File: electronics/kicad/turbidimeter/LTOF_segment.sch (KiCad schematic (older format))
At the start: 3 parts, among them U2 TSL2571FN

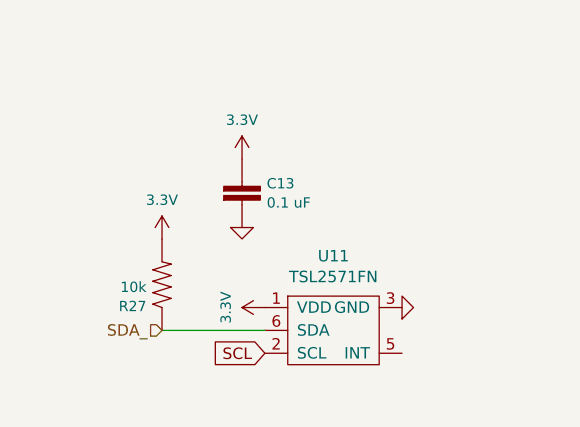
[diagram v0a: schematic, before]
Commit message: turbidimeter
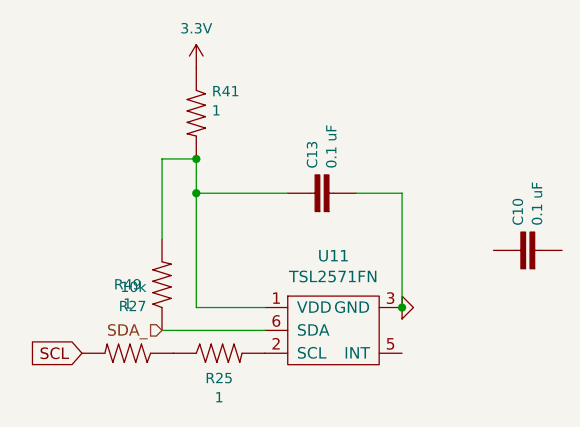
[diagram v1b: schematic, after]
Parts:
- added C3: 0.1 uF, Capacitor_SMD:C_0603_1608Metric, symbol SparkFun-Capacitors:0.1UF-0603-25V-5%
- added R23, R40, R48: 1, 0805, symbol SparkFun-Resistors:RESISTOR0805
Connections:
- net 3.3V: now also R40.1; no longer C4.1, R18.2, U2.1 (VDD)
- net SCL: now also R48.2; no longer U2.2 (SCL)
- new net: C4.1, R18.2, R40.2, U2.1 (VDD)
- new net: R23.2, U2.2 (SCL)
- new net: R23.1, R48.1
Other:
- moved on the sheet: C13
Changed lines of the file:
@@
 $Descr A4 11693 8268
 encoding utf-8
-Sheet 18 33
+Sheet 17 17
 Title ""
 Date ""
@@
 	1    0    0    -1
 $EndComp
-$Comp
-L SparkFun-PowerSymbols:3.3V #SUPPLY?
-U 1 1 5FC4995B
-P 3900 3850
-AR Path="/5FC4995B" Ref="#SUPPLY?"  Part="1"
-AR Path="/5FC47654/5FC4995B" Ref="#SUPPLY0107"  Part="1"
-AR Path="/5FC5771C/5FC4995B" Ref="#SUPPLY0108"  Part="1"
-AR Path="/5FC58972/5FC4995B" Ref="#SUPPLY0109"  Part="1"
-AR Path="/5FC5929A/5FC4995B" Ref="#SUPPLY0110"  Part="1"
-AR Path="/5FC59BFE/5FC4995B" Ref="#SUPPLY?"  Part="1"
-AR Path="/5FC5B14C/5FC4995B" Ref="#SUPPLY0111"  Part="1"
-AR Path="/5FC5B14F/5FC4995B" Ref="#SUPPLY0112"  Part="1"
-AR Path="/5FC5B152/5FC4995B" Ref="#SUPPLY0113"  Part="1"
-AR Path="/5FC5B155/5FC4995B" Ref="#SUPPLY0114"  Part="1"
-AR Path="/5FC5BFFA/5FC4995B" Ref="#SUPPLY0115"  Part="1"
-AR Path="/5FC5BFFD/5FC4995B" Ref="#SUPPLY0116"  Part="1"
-AR Path="/5FC5C000/5FC4995B" Ref="#SUPPLY0117"  Part="1"
-AR Path="/5FC5C003/5FC4995B" Ref="#SUPPLY0118"  Part="1"
-AR Path="/5FC5C006/5FC4995B" Ref="#SUPPLY0119"  Part="1"
-AR Path="/5FC5C009/5FC4995B" Ref="#SUPPLY0120"  Part="1"
-AR Path="/5FC5C00C/5FC4995B" Ref="#SUPPLY0121"  Part="1"
-AR Path="/5FC5C00F/5FC4995B" Ref="#SUPPLY0122"  Part="1"
-F 0 "#SUPPLY0116" H 3950 3850 45  0001 L BNN
-F 1 "3.3V" H 3900 4020 45  0000 C CNN
-F 2 "" V 3858 3977 60  0000 L CNN
-F 3 "" H 3900 3850 60  0001 C CNN
-	1    3900 3850
-	0    -1   -1   0
-$EndComp
-Text GLabel 3900 4050 0    50   Input ~ 0
+Text GLabel 3100 4050 0    50   Input ~ 0
 SCL
 $Comp
@@
 L SparkFun-PowerSymbols:3.3V #SUPPLY?
 U 1 1 5FCB8149
-P 3450 3550
+P 3600 2800
 AR Path="/5FCB8149" Ref="#SUPPLY?"  Part="1"
 AR Path="/5FC47654/5FCB8149" Ref="#SUPPLY0123"  Part="1"
@@
 AR Path="/5FC5C00C/5FCB8149" Ref="#SUPPLY0137"  Part="1"
 AR Path="/5FC5C00F/5FCB8149" Ref="#SUPPLY0138"  Part="1"
-F 0 "#SUPPLY0132" H 3500 3550 45  0001 L BNN
-F 1 "3.3V" H 3450 3720 45  0000 C CNN
-F 2 "" V 3408 3677 60  0000 L CNN
-F 3 "" H 3450 3550 60  0001 C CNN
-	1    3450 3550
+F 0 "#SUPPLY0132" H 3650 2800 45  0001 L BNN
+F 1 "3.3V" H 3600 2970 45  0000 C CNN
+F 2 "" V 3558 2927 60  0000 L CNN
+F 3 "" H 3600 2800 60  0001 C CNN
+	1    3600 2800
 	1    0    0    -1
 $EndComp
 Wire Wire Line
 	3900 3950 3450 3950
-$Comp
-L power:GND #PWR?
-U 1 1 5FCB9EE0
-P 3800 3500
-AR Path="/5FCB9EE0" Ref="#PWR?"  Part="1"
-AR Path="/5FC47654/5FCB9EE0" Ref="#PWR0141"  Part="1"
-AR Path="/5FC5771C/5FCB9EE0" Ref="#PWR0142"  Part="1"
-AR Path="/5FC58972/5FCB9EE0" Ref="#PWR0143"  Part="1"
-AR Path="/5FC5929A/5FCB9EE0" Ref="#PWR0144"  Part="1"
-AR Path="/5FC5B14C/5FCB9EE0" Ref="#PWR0145"  Part="1"
-AR Path="/5FC5B14F/5FCB9EE0" Ref="#PWR0146"  Part="1"
-AR Path="/5FC5B152/5FCB9EE0" Ref="#PWR0147"  Part="1"
-AR Path="/5FC5B155/5FCB9EE0" Ref="#PWR0148"  Part="1"
-AR Path="/5FC5BFFA/5FCB9EE0" Ref="#PWR0149"  Part="1"
-AR Path="/5FC5BFFD/5FCB9EE0" Ref="#PWR0150"  Part="1"
-AR Path="/5FC5C000/5FCB9EE0" Ref="#PWR0151"  Part="1"
-AR Path="/5FC5C003/5FCB9EE0" Ref="#PWR0152"  Part="1"
-AR Path="/5FC5C006/5FCB9EE0" Ref="#PWR0153"  Part="1"
-AR Path="/5FC5C009/5FCB9EE0" Ref="#PWR0154"  Part="1"
-AR Path="/5FC5C00C/5FCB9EE0" Ref="#PWR0155"  Part="1"
-AR Path="/5FC5C00F/5FCB9EE0" Ref="#PWR0156"  Part="1"
-F 0 "#PWR0150" H 3800 3500 30  0001 C CNN
-F 1 "GND" H 3800 3430 30  0001 C CNN
-F 2 "" H 3800 3500 50  0001 C CNN
-F 3 "" H 3800 3500 50  0001 C CNN
-	1    3800 3500
-	1    0    0    -1
-$EndComp
 $Comp
 L SparkFun-Capacitors:0.1UF-0603-25V-5% C?
 U 1 1 5FCB9EE7
-P 3800 3400
+P 4200 3350
 AR Path="/5FCB9EE7" Ref="C?"  Part="1"
 AR Path="/5FC47654/5FCB9EE7" Ref="C4"  Part="1"
@@
 AR Path="/5FC5C00C/5FCB9EE7" Ref="C18"  Part="1"
 AR Path="/5FC5C00F/5FCB9EE7" Ref="C19"  Part="1"
-F 0 "C13" H 3908 3492 45  0000 L CNN
-F 1 "0.1 uF" H 3908 3408 45  0000 L CNN
-F 2 "Capacitor_SMD:C_0603_1608Metric" H 3800 3650 20  0001 C CNN
-F 3 "" H 3800 3400 50  0001 C CNN
-F 4 "" H 3908 3366 60  0000 L CNN "Field4"
-	1    3800 3400
+F 0 "C13" H 4308 3442 45  0000 L CNN
+F 1 "0.1 uF" H 4308 3358 45  0000 L CNN
+F 2 "Capacitor_SMD:C_0603_1608Metric" H 4200 3600 20  0001 C CNN
+F 3 "" H 4200 3350 50  0001 C CNN
+F 4 "" H 4308 3316 60  0000 L CNN "Field4"
+	1    4200 3350
+	0    -1   -1   0
+$EndComp
+Wire Wire Line
+	3450 3550 3450 3200
+$Comp
+L SparkFun-Resistors:RESISTOR0805 R23
+U 1 1 60C85497
+P 3700 4050
+AR Path="/5FC5C00F/60C85497" Ref="R23"  Part="1"
+AR Path="/5FC5BFFA/60C85497" Ref="R10"  Part="1"
+AR Path="/5FC5C000/60C85497" Ref="R12"  Part="1"
+AR Path="/5FC5C003/60C85497" Ref="R14"  Part="1"
+AR Path="/5FC5C006/60C85497" Ref="R16"  Part="1"
+AR Path="/5FC5C009/60C85497" Ref="R19"  Part="1"
+AR Path="/5FC5C00C/60C85497" Ref="R21"  Part="1"
+AR Path="/5FC5BFFD/60C85497" Ref="R25"  Part="1"
+F 0 "R25" H 3700 3940 45  0000 C CNN
+F 1 "1" H 3700 3856 45  0000 C CNN
+F 2 "0805" H 3700 4200 20  0001 C CNN
+F 3 "" H 3700 4050 60  0001 C CNN
+F 4 " " H 3700 3761 60  0000 C CNN "Field4"
+	1    3700 4050
 	1    0    0    -1
 $EndComp
-$Comp
-L SparkFun-PowerSymbols:3.3V #SUPPLY?
-U 1 1 5FCB9F0F
-P 3800 3200
-AR Path="/5FCB9F0F" Ref="#SUPPLY?"  Part="1"
-AR Path="/5FC47654/5FCB9F0F" Ref="#SUPPLY0139"  Part="1"
-AR Path="/5FC5771C/5FCB9F0F" Ref="#SUPPLY0140"  Part="1"
-AR Path="/5FC58972/5FCB9F0F" Ref="#SUPPLY0141"  Part="1"
-AR Path="/5FC5929A/5FCB9F0F" Ref="#SUPPLY0142"  Part="1"
-AR Path="/5FC59BFE/5FCB9F0F" Ref="#SUPPLY?"  Part="1"
-AR Path="/5FC5B14C/5FCB9F0F" Ref="#SUPPLY0143"  Part="1"
-AR Path="/5FC5B14F/5FCB9F0F" Ref="#SUPPLY0144"  Part="1"
-AR Path="/5FC5B152/5FCB9F0F" Ref="#SUPPLY0145"  Part="1"
-AR Path="/5FC5B155/5FCB9F0F" Ref="#SUPPLY0146"  Part="1"
-AR Path="/5FC5BFFA/5FCB9F0F" Ref="#SUPPLY0147"  Part="1"
-AR Path="/5FC5BFFD/5FCB9F0F" Ref="#SUPPLY0148"  Part="1"
-AR Path="/5FC5C000/5FCB9F0F" Ref="#SUPPLY0149"  Part="1"
-AR Path="/5FC5C003/5FCB9F0F" Ref="#SUPPLY0150"  Part="1"
-AR Path="/5FC5C006/5FCB9F0F" Ref="#SUPPLY0151"  Part="1"
-AR Path="/5FC5C009/5FCB9F0F" Ref="#SUPPLY0152"  Part="1"
-AR Path="/5FC5C00C/5FCB9F0F" Ref="#SUPPLY0153"  Part="1"
-AR Path="/5FC5C00F/5FCB9F0F" Ref="#SUPPLY0154"  Part="1"
-F 0 "#SUPPLY0148" H 3850 3200 45  0001 L BNN
-F 1 "3.3V" H 3800 3370 45  0000 C CNN
-F 2 "" V 3758 3327 60  0000 L CNN
-F 3 "" H 3800 3200 60  0001 C CNN
-	1    3800 3200
-	1    0    0    -1
-$EndComp
+Wire Wire Line
+	3600 3850 3900 3850
+Wire Wire Line
+	4500 3850 4500 3350
+Wire Wire Line
+	4500 3350 4300 3350
+Wire Wire Line
+	3600 3350 3600 3850
+Connection ~ 3600 3350
+Wire Wire Line
+	4000 3350 3600 3350
+Wire Wire Line
+	3600 3200 3600 3350
+$Comp
+L SparkFun-Resistors:RESISTOR0805 R48
+U 1 1 60C907D0
+P 3300 4050
+AR Path="/5FC5C00F/60C907D0" Ref="R48"  Part="1"
+AR Path="/5FC5BFFA/60C907D0" Ref="R42"  Part="1"
+AR Path="/5FC5C000/60C907D0" Ref="R43"  Part="1"
+AR Path="/5FC5C003/60C907D0" Ref="R44"  Part="1"
+AR Path="/5FC5C006/60C907D0" Ref="R45"  Part="1"
+AR Path="/5FC5C009/60C907D0" Ref="R46"  Part="1"
+AR Path="/5FC5C00C/60C907D0" Ref="R47"  Part="1"
+AR Path="/5FC5BFFD/60C907D0" Ref="R49"  Part="1"
+F 0 "R49" H 3300 3750 45  0000 C CNN
+F 1 "1" H 3300 3834 45  0000 C CNN
+F 2 "0805" H 3300 4200 20  0001 C CNN
+F 3 "" H 3300 4050 60  0001 C CNN
+F 4 " " H 3300 3929 60  0000 C CNN "Field4"
+	1    3300 4050
+	-1   0    0    1
+$EndComp
+Wire Wire Line
+	3450 3200 3600 3200
+Connection ~ 4500 3850
+$Comp
+L SparkFun-Capacitors:0.1UF-0603-25V-5% C?
+U 1 1 60C96374
+P 5100 3600
+AR Path="/60C96374" Ref="C?"  Part="1"
+AR Path="/5FC47654/60C96374" Ref="C?"  Part="1"
+AR Path="/5FC5771C/60C96374" Ref="C?"  Part="1"
+AR Path="/5FC58972/60C96374" Ref="C?"  Part="1"
+AR Path="/5FC5929A/60C96374" Ref="C?"  Part="1"
+AR Path="/5FC5B14C/60C96374" Ref="C?"  Part="1"
+AR Path="/5FC5B14F/60C96374" Ref="C?"  Part="1"
+AR Path="/5FC5B152/60C96374" Ref="C?"  Part="1"
+AR Path="/5FC5B155/60C96374" Ref="C?"  Part="1"
+AR Path="/5FC5BFFA/60C96374" Ref="C3"  Part="1"
+AR Path="/5FC5BFFD/60C96374" Ref="C10"  Part="1"
+AR Path="/5FC5C000/60C96374" Ref="C4"  Part="1"
+AR Path="/5FC5C003/60C96374" Ref="C5"  Part="1"
+AR Path="/5FC5C006/60C96374" Ref="C6"  Part="1"
+AR Path="/5FC5C009/60C96374" Ref="C7"  Part="1"
+AR Path="/5FC5C00C/60C96374" Ref="C8"  Part="1"
+AR Path="/5FC5C00F/60C96374" Ref="C9"  Part="1"
+F 0 "C10" H 5208 3692 45  0000 L CNN
+F 1 "0.1 uF" H 5208 3608 45  0000 L CNN
+F 2 "Capacitor_SMD:C_0603_1608Metric" H 5100 3850 20  0001 C CNN
+F 3 "" H 5100 3600 50  0001 C CNN
+F 4 "" H 5208 3566 60  0000 L CNN "Field4"
+	1    5100 3600
+	0    -1   -1   0
+$EndComp
+$Comp
+L SparkFun-Resistors:RESISTOR0805 R40
+U 1 1 60C97D01
+P 3600 3000
+AR Path="/5FC5C00F/60C97D01" Ref="R40"  Part="1"
+AR Path="/5FC5BFFA/60C97D01" Ref="R34"  Part="1"
+AR Path="/5FC5C000/60C97D01" Ref="R35"  Part="1"
+AR Path="/5FC5C003/60C97D01" Ref="R36"  Part="1"
+AR Path="/5FC5C006/60C97D01" Ref="R37"  Part="1"
+AR Path="/5FC5C009/60C97D01" Ref="R38"  Part="1"
+AR Path="/5FC5C00C/60C97D01" Ref="R39"  Part="1"
+AR Path="/5FC5BFFD/60C97D01" Ref="R41"  Part="1"
+F 0 "R41" V 3505 3068 45  0000 L CNN
+F 1 "1" V 3589 3068 45  0000 L CNN
+F 2 "0805" H 3600 3150 20  0001 C CNN
+F 3 "" H 3600 3000 60  0001 C CNN
+F 4 " " V 3684 3068 60  0000 L CNN "Field4"
+	1    3600 3000
+	0    1    1    0
+$EndComp
+Connection ~ 3600 3200
 $EndSCHEMATC
